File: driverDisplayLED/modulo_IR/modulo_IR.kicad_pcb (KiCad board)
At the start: 2 copper layers, 15 parts, among them J1 Conn_01x03_Male, U1 SFH617A-1X001, U2 LM393

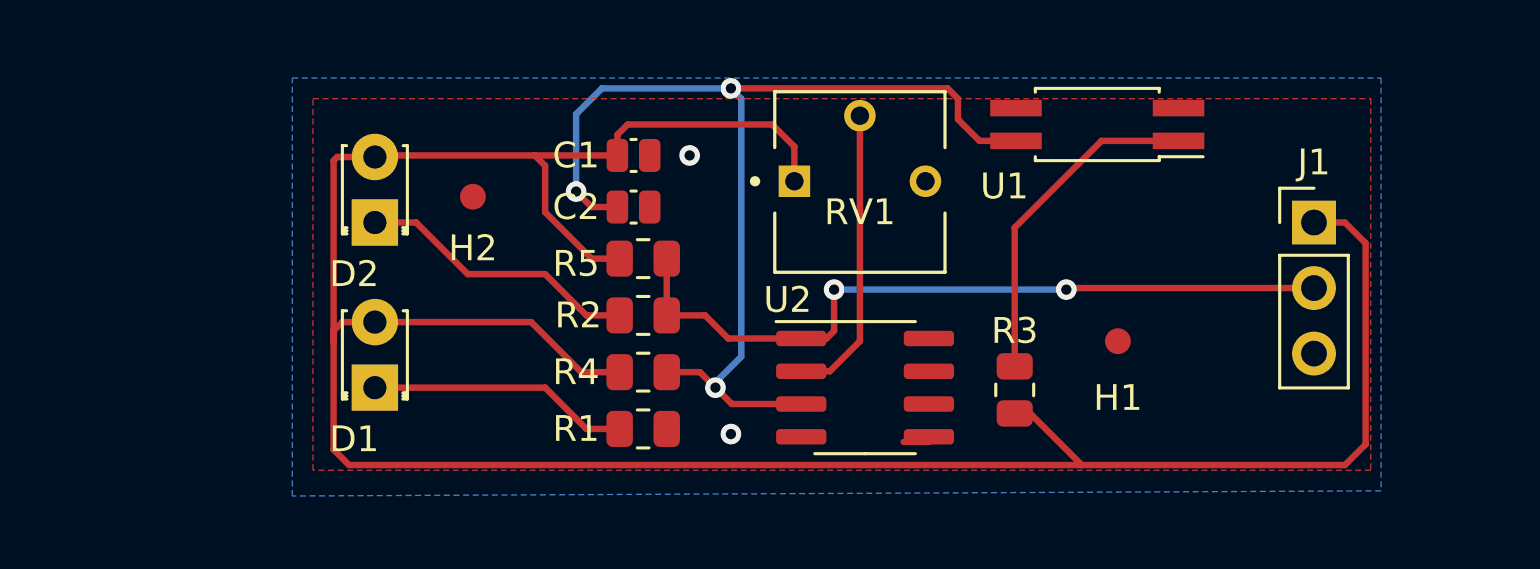
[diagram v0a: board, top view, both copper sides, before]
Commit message: rediseño PCB
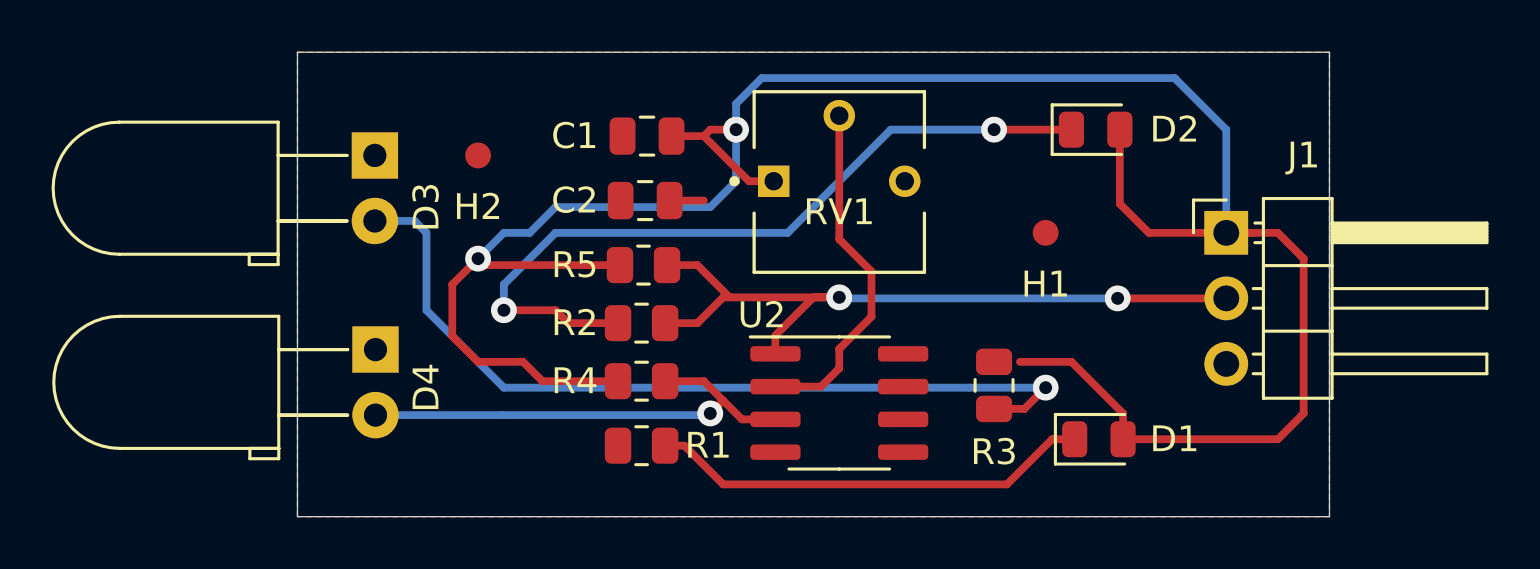
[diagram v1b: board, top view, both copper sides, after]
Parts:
- removed U1: SFH617A-1X001, Package_SO:SO-4_4.4x2.3mm_P1.27mm
- added D3: LED, LED_THT:LED_D5.0mm_Horizontal_O3.81mm_Z3.0mm, F.Cu at (111.0, 77.0)
- added D4: D_Photo, LED_THT:LED_D5.0mm_Horizontal_O3.81mm_Z3.0mm, F.Cu at (111.0, 84.5)
- C1, C2: footprint Capacitor_SMD:C_0504_1310Metric_Pad0.83x1.28mm_HandSolder -> Capacitor_SMD:C_0805_2012Metric
- D1, D2: footprint LED_THT:LED_D1.8mm_W3.3mm_H2.4mm -> Diode_SMD:D_0805_2012Metric
- J1: footprint Connector_PinHeader_2.54mm:PinHeader_1x03_P2.54mm_Vertical -> Connector_PinHeader_2.54mm:PinHeader_1x03_P2.54mm_Horizontal
- moved D2 28.2 mm to (138.9, 76.0), turned to 0 degrees
- moved D1 28.1 mm to (139.1, 88.0), turned to 0 degrees
- moved H1 5.05 mm to (137.0, 80.0)
- moved J1 3.42 mm to (144.0, 80.0)
- moved H2 1.61 mm to (115.0, 77.0)
- moved U2 1.16 mm to (129.0, 86.6)
- moved C1 0.91 mm to (121.5, 76.2), turned to 180 degrees
- moved R3 0.82 mm to (135.0, 85.9), turned to 270 degrees
- moved RV1 0.80 mm to (129.0, 78.0)
- moved R1 0.65 mm to (121.3, 88.2), turned to 180 degrees
- moved C2 0.51 mm to (121.5, 78.8), turned to 180 degrees
- moved R4 0.36 mm to (121.3, 85.8)
- moved R2 0.31 mm to (121.3, 83.5)
- moved R5 0.25 mm to (121.4, 81.2)
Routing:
- net Net-(C2-Pad1): track 41.5 -> 19.9 mm, vias 3 -> 1
- net Net-(D3-Pad2): track 13.1 -> 32.8 mm, vias 0 -> 1
- net Net-(D2-Pad1): track 11.0 -> 30.1 mm, vias 0 -> 2
- net +5V: track 104.4 -> 91.8 mm, vias 0 -> 2
- net Net-(D1-Pad1): track 10.2 -> 17.2 mm
- net Net-(RV1-Pad2): track 11.5 -> 13.6 mm
- net (no net): track 0.98 -> 0.00 mm
- net GND: vias 2 -> 0
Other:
- board outline added: 40 x 18 mm
- rule trace_min: 0.2 -> 0.3
- rule via_min_size: 0.4 -> 0.5

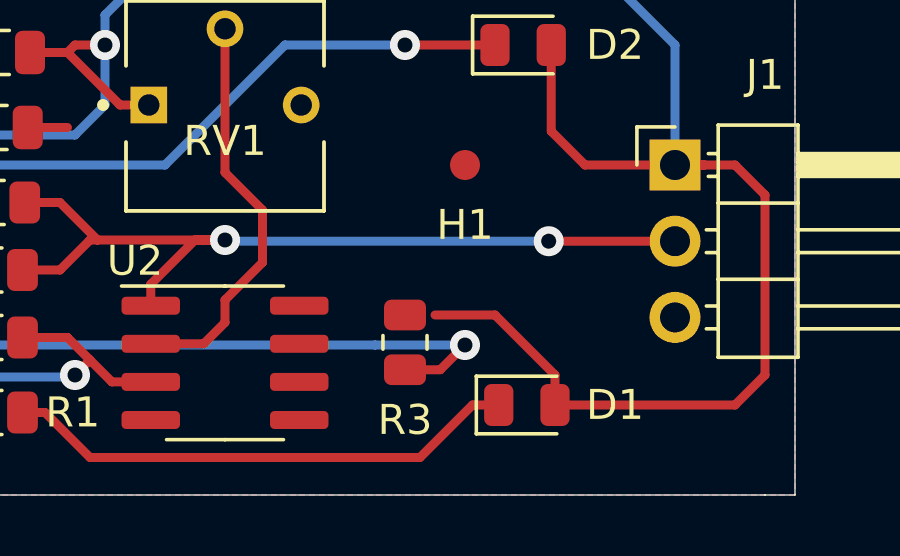
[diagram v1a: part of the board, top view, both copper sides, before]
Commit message: rediseño PCB
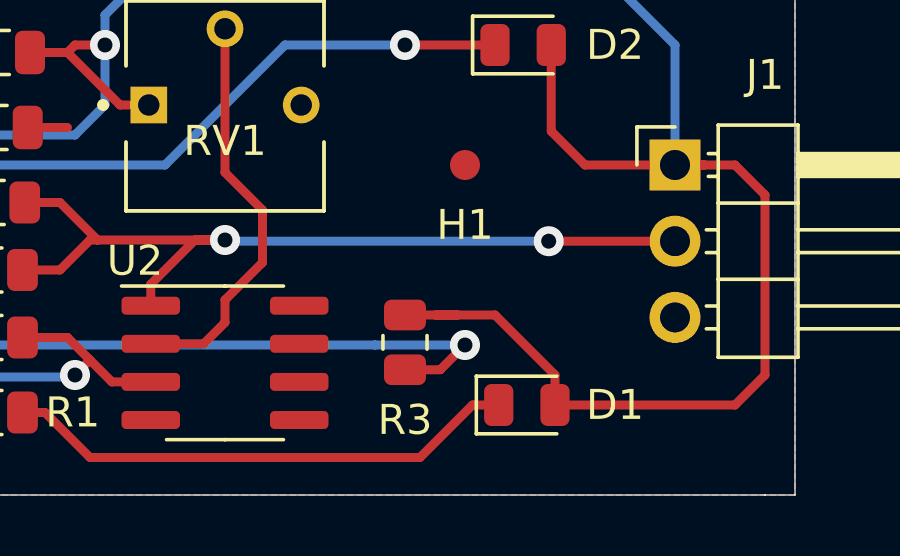
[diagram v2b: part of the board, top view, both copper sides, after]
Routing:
- net +5V: track 91.8 -> 93.6 mm
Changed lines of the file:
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@@
     (thickness 1.6)
     (drawings 5)
-    (tracks 95)
+    (tracks 97)
     (zones 0)
     (modules 16)
@@
   (segment (start 123.75 76.25) (end 122.5 76.25) (width 0.3) (layer F.Cu) (net 1))
   (segment (start 140 88) (end 140 87) (width 0.3) (layer F.Cu) (net 1))
-  (segment (start 138 85) (end 136 85) (width 0.3) (layer F.Cu) (net 1))
   (segment (start 140 87) (end 138 85) (width 0.3) (layer F.Cu) (net 1))
   (via (at 125 76) (size 1) (drill 0.5) (layers F.Cu B.Cu) (net 1))
@@
   (segment (start 114 82) (end 115 81) (width 0.3) (layer F.Cu) (net 1))
   (segment (start 114 84) (end 114 82) (width 0.3) (layer F.Cu) (net 1))
+  (segment (start 136.75 85) (end 135 85) (width 0.3) (layer F.Cu) (net 1))
+  (segment (start 138 85) (end 136.75 85) (width 0.3) (layer F.Cu) (net 1))
+  (segment (start 136.75 85) (end 136 85) (width 0.3) (layer F.Cu) (net 1))
   (segment (start 126.525 87.23) (end 125.23 87.23) (width 0.3) (layer F.Cu) (net 3))
   (segment (start 123.75 85.75) (end 122.25 85.75) (width 0.3) (layer F.Cu) (net 3))
